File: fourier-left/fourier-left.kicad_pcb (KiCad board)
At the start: 2 copper layers, 124.4 x 80.4 mm, 129 parts, among them J1 VCC, J3 RGB, J6 C6, J7 GND, U1 ProMicro, U2 TRRS

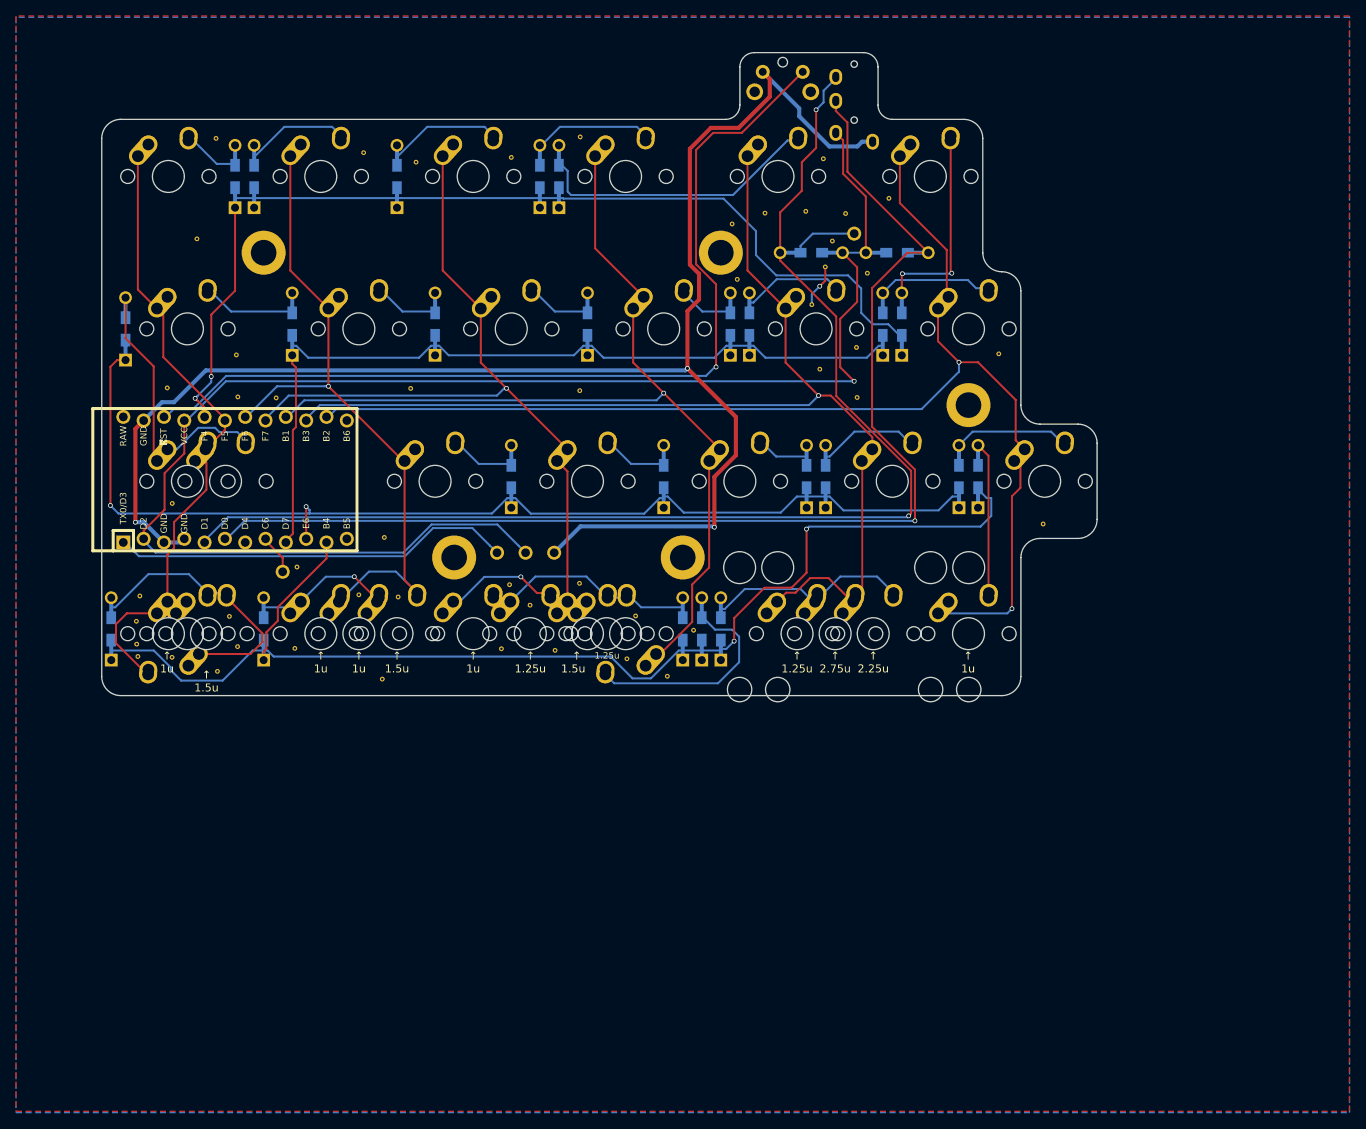
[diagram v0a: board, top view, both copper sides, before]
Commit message: adad
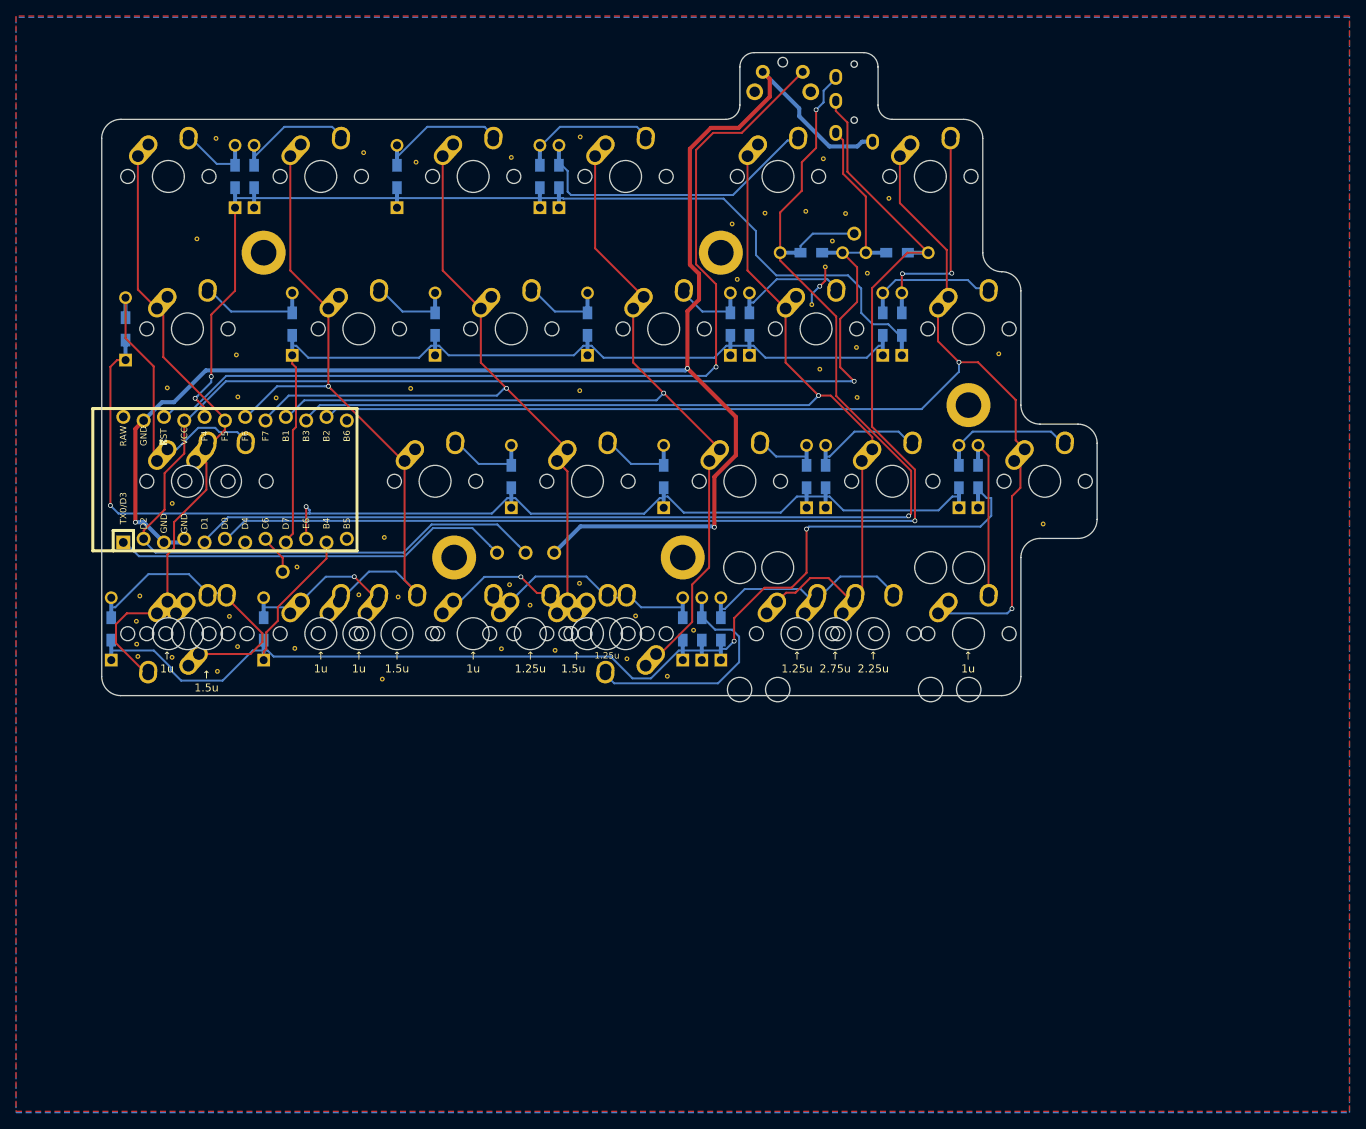
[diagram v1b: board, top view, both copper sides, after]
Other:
- net class Default removed
- net class Power removed
